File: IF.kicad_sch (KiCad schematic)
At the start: 34 parts, among them J10 AudioJack3_Ground_SwitchTR, K1 RS-12, Q9 MMBT2222A, U5 MC33079

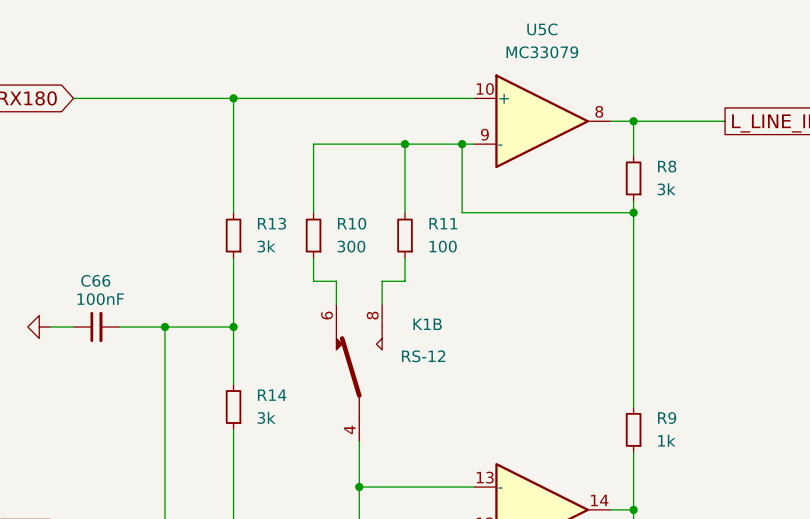
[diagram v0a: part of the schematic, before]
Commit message: progress on PCB
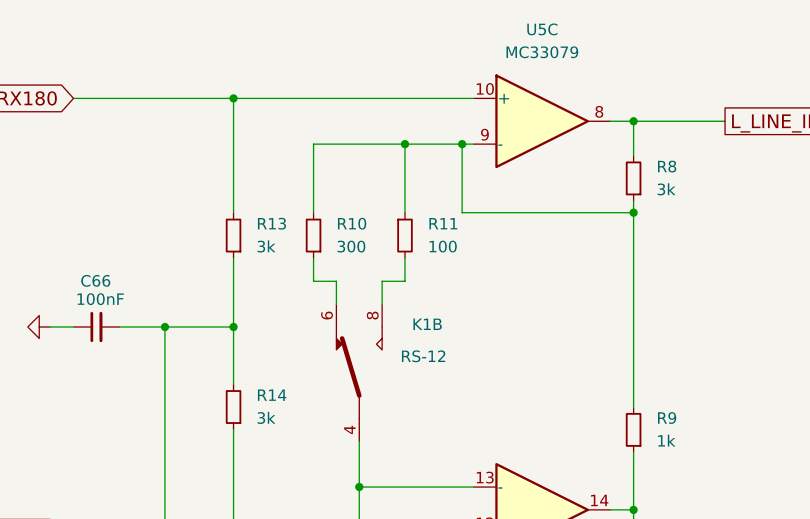
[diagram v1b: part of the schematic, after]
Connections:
- net at R10.2, R8.1, R9.2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: now also R11.1; no longer R11.2
- net at K1.8: now also R11.2; no longer R11.1
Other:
- moved on the sheet: R11
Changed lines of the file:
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@@
 	(symbol
 		(lib_id "Device:R_Small")
-		(at 78.74 45.72 180)
+		(at 78.74 45.72 0)
 		(unit 1)
 		(exclude_from_sim no)
@@
 					(size 1.27 1.27)
 				)
-				(justify right)
+				(justify left)
 			)
 		)
@@
 					(size 1.27 1.27)
 				)
-				(justify right)
+				(justify left)
 			)
 		)
